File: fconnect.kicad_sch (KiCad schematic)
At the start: 198 parts, among them J1 9001-11961C00A, J2 9001-11961C00A, J3 7760, J4 7760

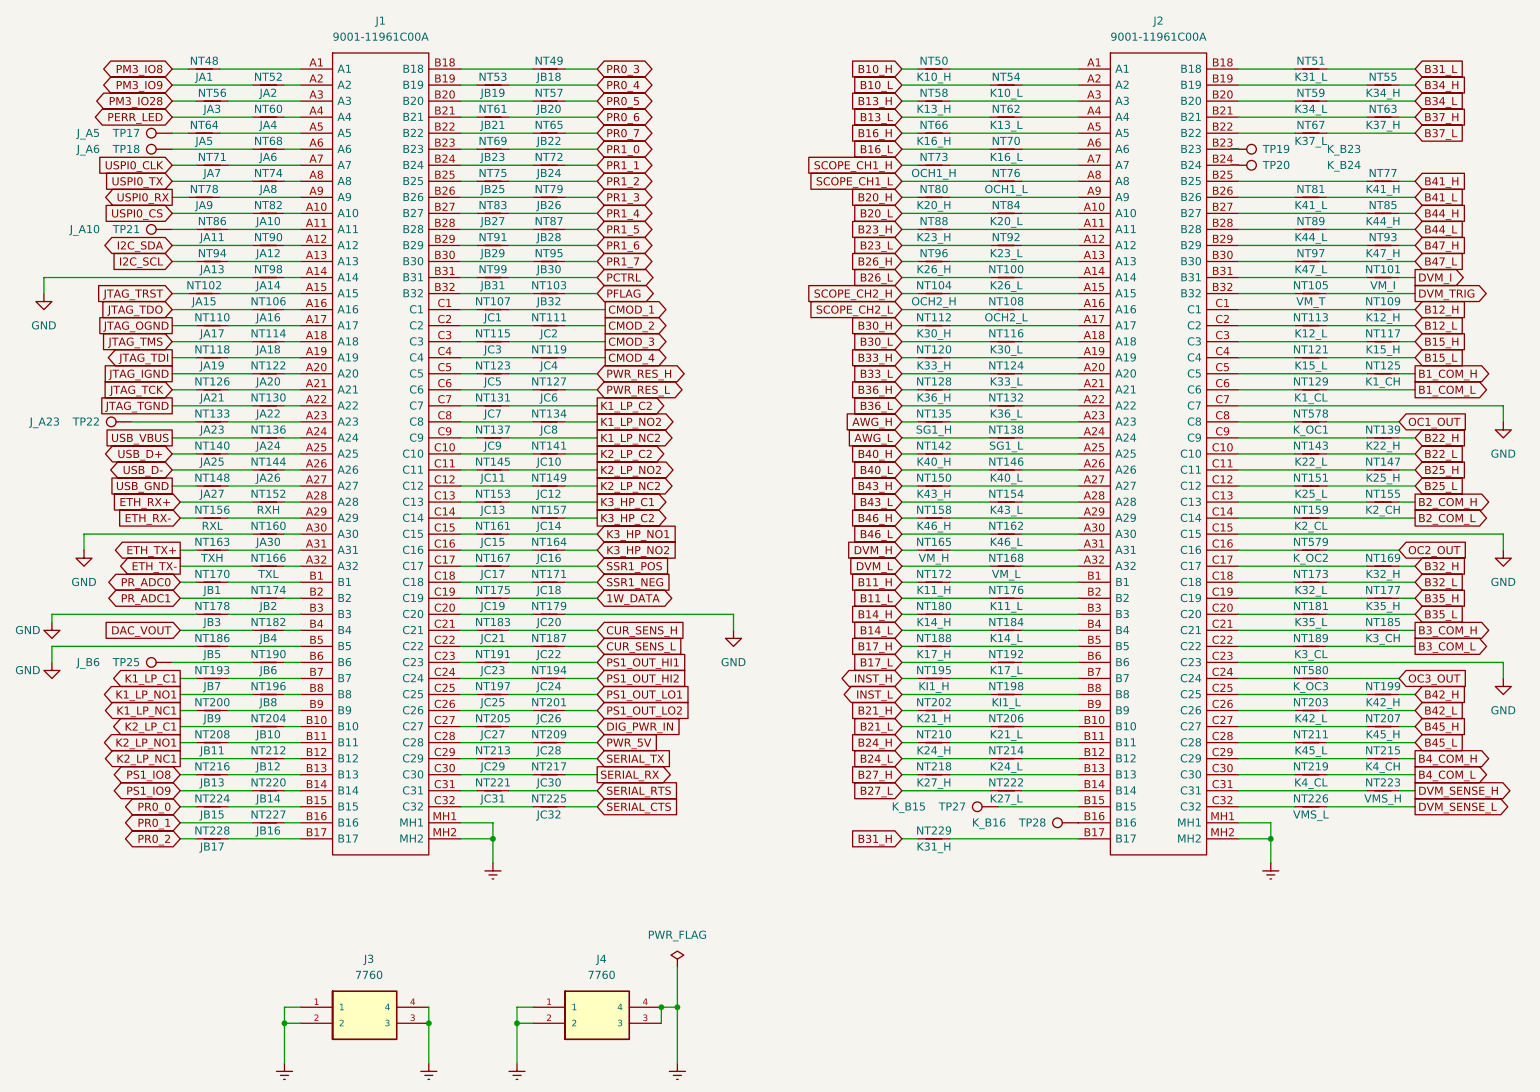
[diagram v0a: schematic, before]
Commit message: First try to fit electronic on PCB
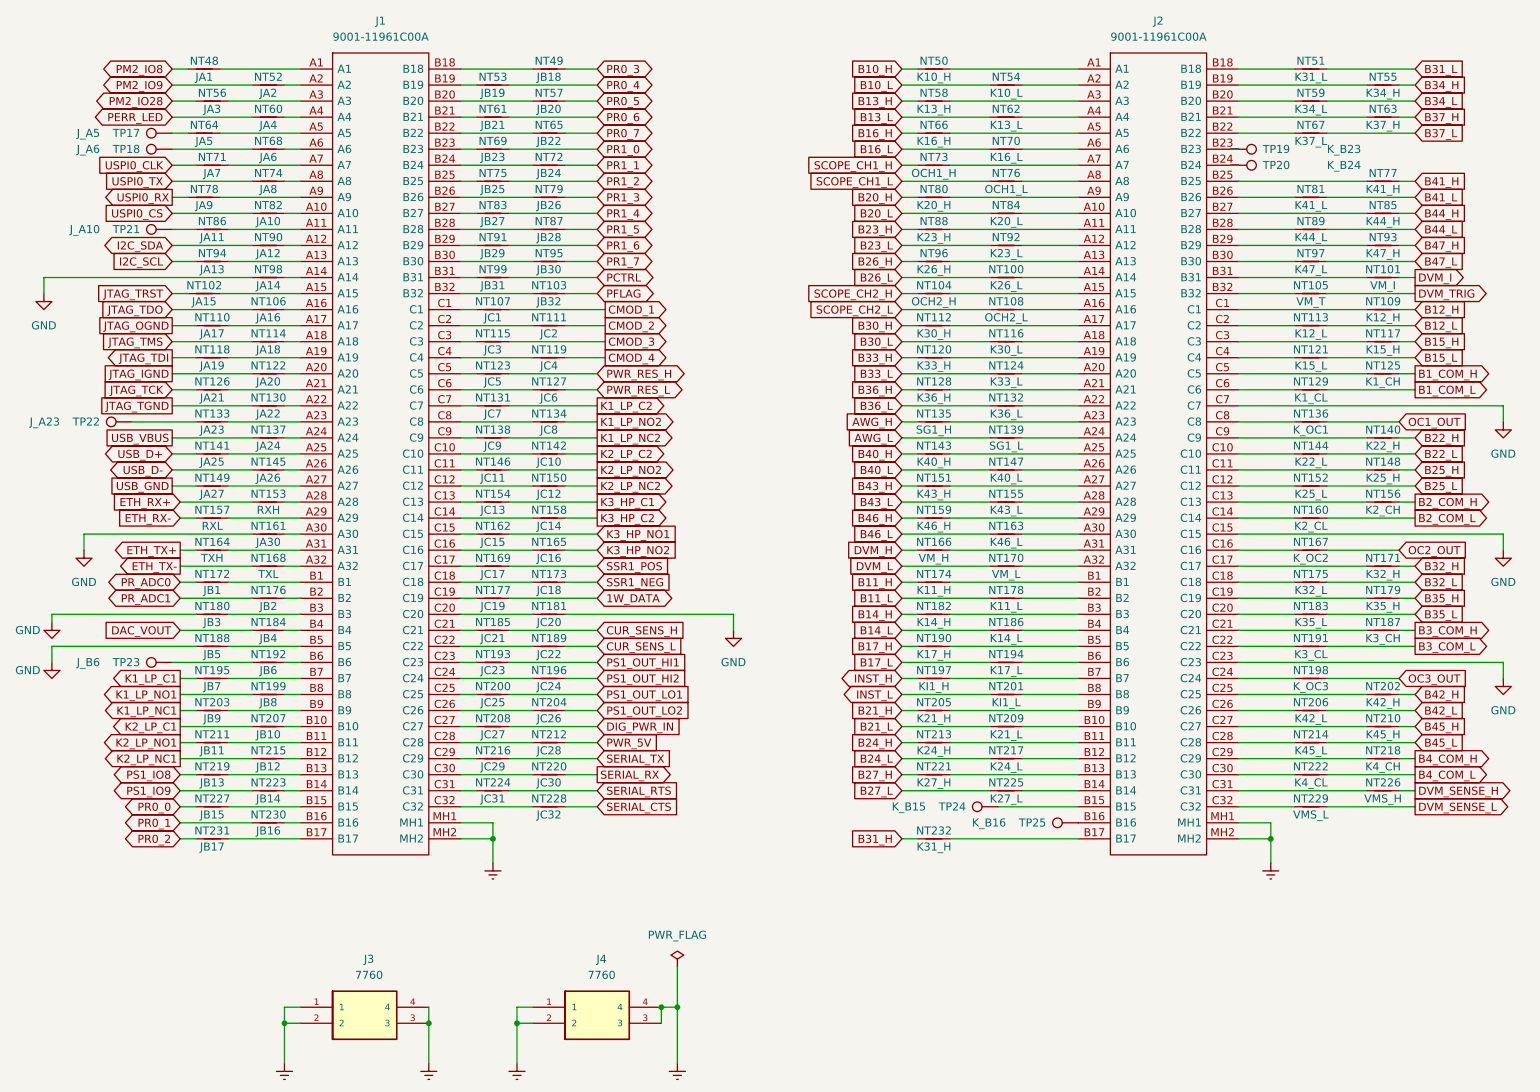
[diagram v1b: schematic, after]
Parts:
- TP17, TP18, TP19, TP20, TP21, TP22: footprint Connector_Pin:Pin_D1.2mm_L11.3mm_W3.0mm_Flat -> Connector_Pin:Pin_D1.0mm_L10.0mm
- TP23: renamed from TP25; footprint Connector_Pin:Pin_D1.2mm_L11.3mm_W3.0mm_Flat -> Connector_Pin:Pin_D1.0mm_L10.0mm
- TP24: renamed from TP27; footprint Connector_Pin:Pin_D1.2mm_L11.3mm_W3.0mm_Flat -> Connector_Pin:Pin_D1.0mm_L10.0mm
- TP25: renamed from TP28; footprint Connector_Pin:Pin_D1.2mm_L11.3mm_W3.0mm_Flat -> Connector_Pin:Pin_D1.0mm_L10.0mm
- renumbered NT578 to NT136, NT136 to NT137, NT137 to NT138, NT138 to NT139, NT139 to NT140, NT140 to NT141, NT141 to NT142, NT142 to NT143, NT143 to NT144, NT144 to NT145, NT145 to NT146, NT146 to NT147, NT147 to NT148, NT148 to NT149, NT149 to NT150, NT150 to NT151, NT151 to NT152, NT152 to NT153, NT153 to NT154, NT154 to NT155, NT155 to NT156, NT156 to NT157, NT157 to NT158, NT158 to NT159, NT159 to NT160, NT160 to NT161, NT161 to NT162, NT162 to NT163, NT163 to NT164, NT164 to NT165, NT165 to NT166, NT579 to NT167, NT166 to NT168, NT167 to NT169, NT168 to NT170, NT169 to NT171, NT170 to NT172, NT171 to NT173, NT172 to NT174, NT173 to NT175, NT174 to NT176, NT175 to NT177, NT176 to NT178, NT177 to NT179, NT178 to NT180, NT179 to NT181, NT180 to NT182, NT181 to NT183, NT182 to NT184, NT183 to NT185, NT184 to NT186, NT185 to NT187, NT186 to NT188, NT187 to NT189, NT188 to NT190, NT189 to NT191, NT190 to NT192, NT191 to NT193, NT192 to NT194, NT193 to NT195, NT194 to NT196, NT195 to NT197, NT580 to NT198, NT196 to NT199, NT197 to NT200, NT198 to NT201, NT199 to NT202, NT200 to NT203, NT201 to NT204, NT202 to NT205, NT203 to NT206, NT204 to NT207, NT205 to NT208, NT206 to NT209, NT207 to NT210, NT208 to NT211, NT209 to NT212, NT210 to NT213, NT211 to NT214, NT212 to NT215, NT213 to NT216, NT214 to NT217, NT215 to NT218, NT216 to NT219, NT217 to NT220, NT218 to NT221, NT219 to NT222, NT220 to NT223, NT221 to NT224, NT222 to NT225, NT223 to NT226, NT224 to NT227, NT225 to NT228, NT226 to NT229, NT227 to NT230, NT228 to NT231, NT229 to NT232
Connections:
- net PM3_IO28 renamed PM2_IO28
- net PM3_IO8 renamed PM2_IO8
- net PM3_IO9 renamed PM2_IO9

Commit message: backup 1 bank done
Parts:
- NT100, NT101, NT102, NT103, NT104, NT105, NT106, NT107, NT108, NT109, NT110, NT111, NT112, NT113, NT114, NT115, NT116, NT117, NT118, NT119, NT120, NT121, NT122, NT123, NT124, NT125, NT126, NT127, NT128, NT129, NT130, NT131, NT132, NT133, NT134, NT135, NT136, NT137, NT138, NT139, NT140, NT141, NT142, NT143, NT144, NT145, NT146, NT147, NT148, NT149, NT150, NT151, NT152, NT153, NT154, NT155, NT156, NT157, NT158, NT159, NT160, NT161, NT162, NT163, NT164, NT165, NT166, NT167, NT168, NT169, NT170, NT171, NT172, NT173, NT174, NT175, NT176, NT177, NT178, NT179, NT180, NT181, NT182, NT183, NT184, NT185, NT186, NT187, NT188, NT189, NT190, NT191, NT192, NT193, NT194, NT195, NT196, NT197, NT198, NT199, NT200, NT201, NT202, NT203, NT204, NT205, NT206, NT207, NT208, NT209, NT210, NT211, NT212, NT213, NT214, NT215, NT216, NT217, NT218, NT219, NT220, NT221, NT222, NT223, NT224, NT225, NT226, NT227, NT228, NT229, NT230, NT231, NT232, NT48, NT49, NT50, NT51, NT52, NT53, NT54, NT55, NT56, NT57, NT58, NT59, NT60, NT61, NT62, NT63, NT64, NT65, NT66, NT67, NT68, NT69, NT70, NT71, NT72, NT73, NT74, NT75, NT76, NT77, NT78, NT79, NT80, NT81, NT82, NT83, NT84, NT85, NT86, NT87, NT88, NT89, NT90, NT91, NT92, NT93, NT94, NT95, NT96, NT97, NT98, NT99: footprint NetTie:NetTie-2_THT_Pad1.0mm -> NetTie:NetTie-2_Front1.0mm
- TP17, TP18, TP19, TP20, TP21, TP22, TP23, TP24, TP25: footprint Connector_Pin:Pin_D1.0mm_L10.0mm -> Connector_Pin:Pin_D0.9mm_L10.0mm_W2.4mm_FlatFork
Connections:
- net AWG_H: now also NT135.2; no longer NT135.1
- net AWG_L: now also NT139.2; no longer NT139.1
- net SCOPE_CH1_H: now also NT73.2; no longer NT73.1
- net SCOPE_CH1_L: now also NT76.2; no longer NT76.1
- net at J2.A7: now also NT73.1; no longer NT73.2
- net at J2.A24: now also NT139.1; no longer NT139.2
- net at J2.A23: now also NT135.1; no longer NT135.2
- net at J2.A8: now also NT76.1; no longer NT76.2
